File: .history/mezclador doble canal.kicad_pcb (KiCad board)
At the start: 2 copper layers, 56.7 x 63.9 mm, 31 parts, among them J1 Conn_Coaxial, J2 Conn_Coaxial, J3 Conn_Coaxial, J4 Conn_Coaxial, J5 Conn_Coaxial, J6 Conn_Coaxial, J7 Screw_Terminal_01x02, U1 NE5532

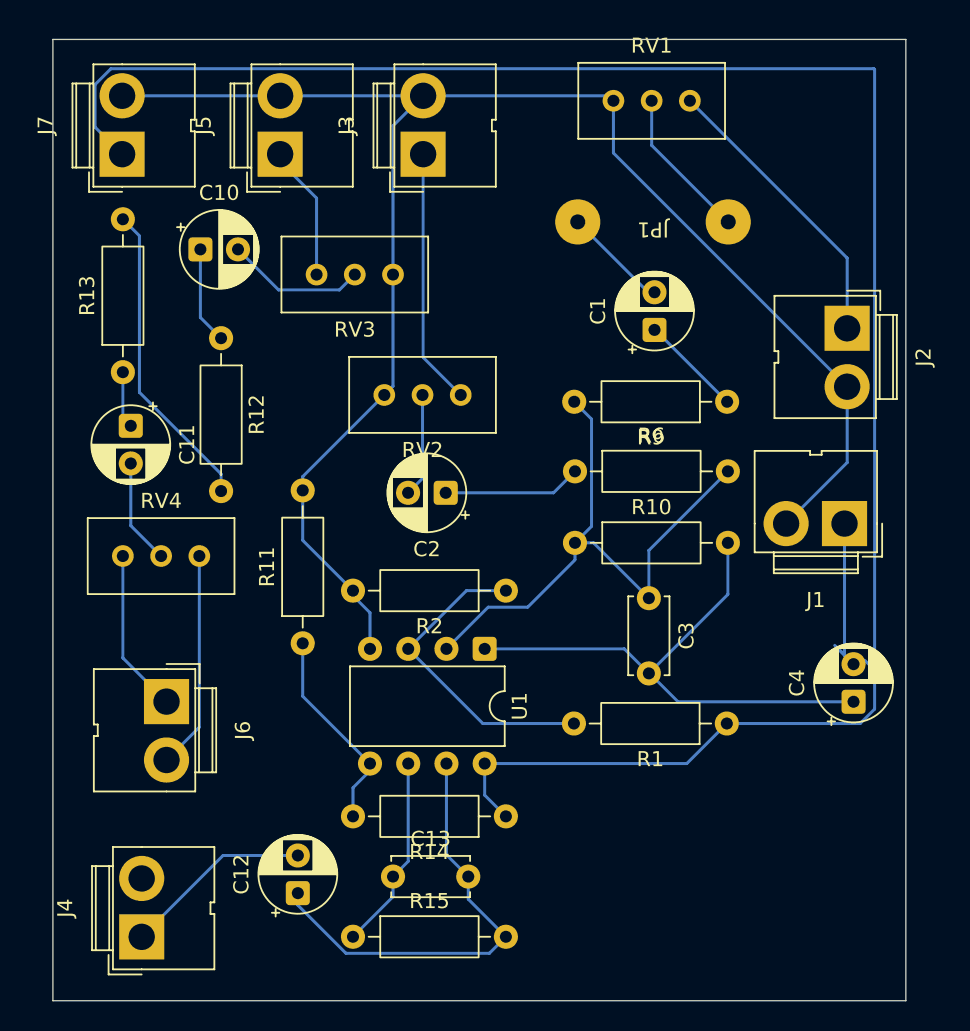
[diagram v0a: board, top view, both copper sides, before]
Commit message: acomodando componentes
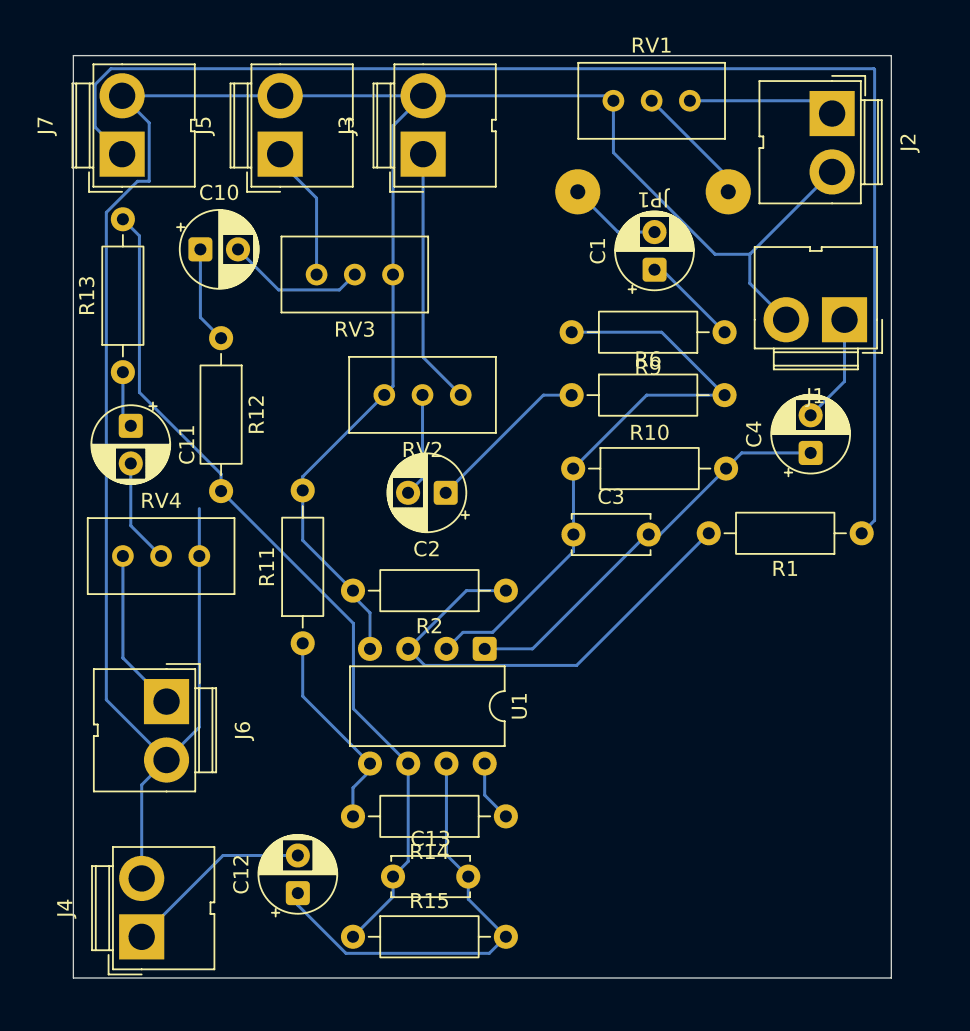
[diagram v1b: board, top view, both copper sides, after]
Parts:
- moved C4 16.8 mm to (222.2, 70.3)
- moved R1 15.5 mm to (225.6, 75.7)
- moved J2 14.3 mm to (223.7, 47.8)
- moved J1 13.5 mm to (224.5, 61.5)
- moved C3 6.56 mm to (206.5, 75.8), turned to 0 degrees
- moved R6 5.07 mm to (206.4, 66.5)
- moved R10 4.94 mm to (206.5, 71.4)
- moved R9 4.62 mm to (216.5, 62.3)
- moved C1 4.00 mm to (211.9, 58.2)
- moved JP1 2.00 mm to (211.8, 53.0)
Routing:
- net GND: track 125.4 -> 177.4 mm
- net VCC: track 131.6 -> 92.9 mm
- net Net-(U1B--): track 33.8 -> 57.0 mm
- net Net-(U1A-+): track 21.2 -> 32.2 mm
- net Net-(J2-In): track 19.4 -> 10.0 mm
- net Net-(C3-Pad2): track 36.8 -> 27.5 mm
- net Net-(J1-In): track 13.3 -> 7.28 mm
- net Net-(JP1-A): track 10.2 -> 8.16 mm
- net Net-(C2-Pad1): track 9.34 -> 11.1 mm
- net Net-(U1A--): track 39.5 -> 40.6 mm
- net Net-(JP1-B): track 7.04 -> 6.21 mm
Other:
- board size 56.7 x 63.9 mm -> 54.4 x 61.3 mm
